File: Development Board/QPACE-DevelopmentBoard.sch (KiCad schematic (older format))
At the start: 25 parts, among them J1 Barrel_Jack_Switch, J10 SWD_ext, J13 RF_External, J2 5Vin-USB, J3 Vin, J4 Vin, J5 RPi_COMPort, J6 WTC_I2C-BUS, J7 Vout, J8 Vout, J9 GPS, SW2 SW_SPDT, U1 BMG160

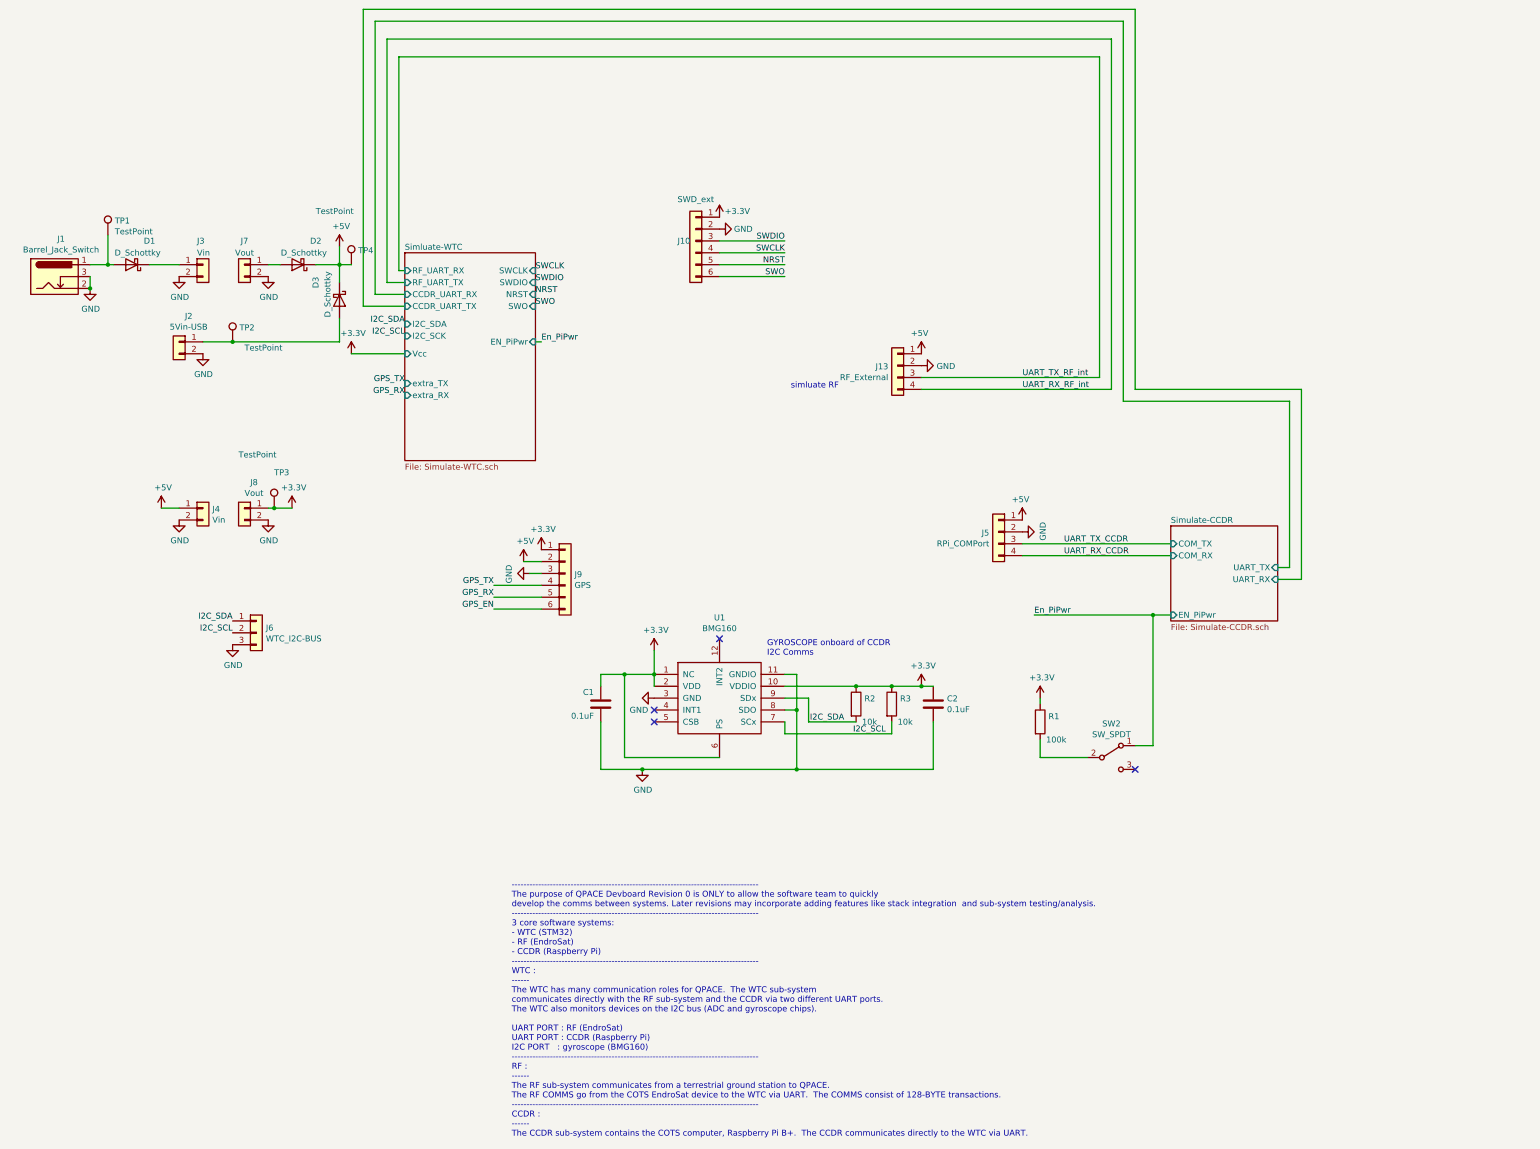
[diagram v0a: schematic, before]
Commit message: ready for production
passed all KiCad error checking. schematic and pcblayout were both validated. ready to be ordered
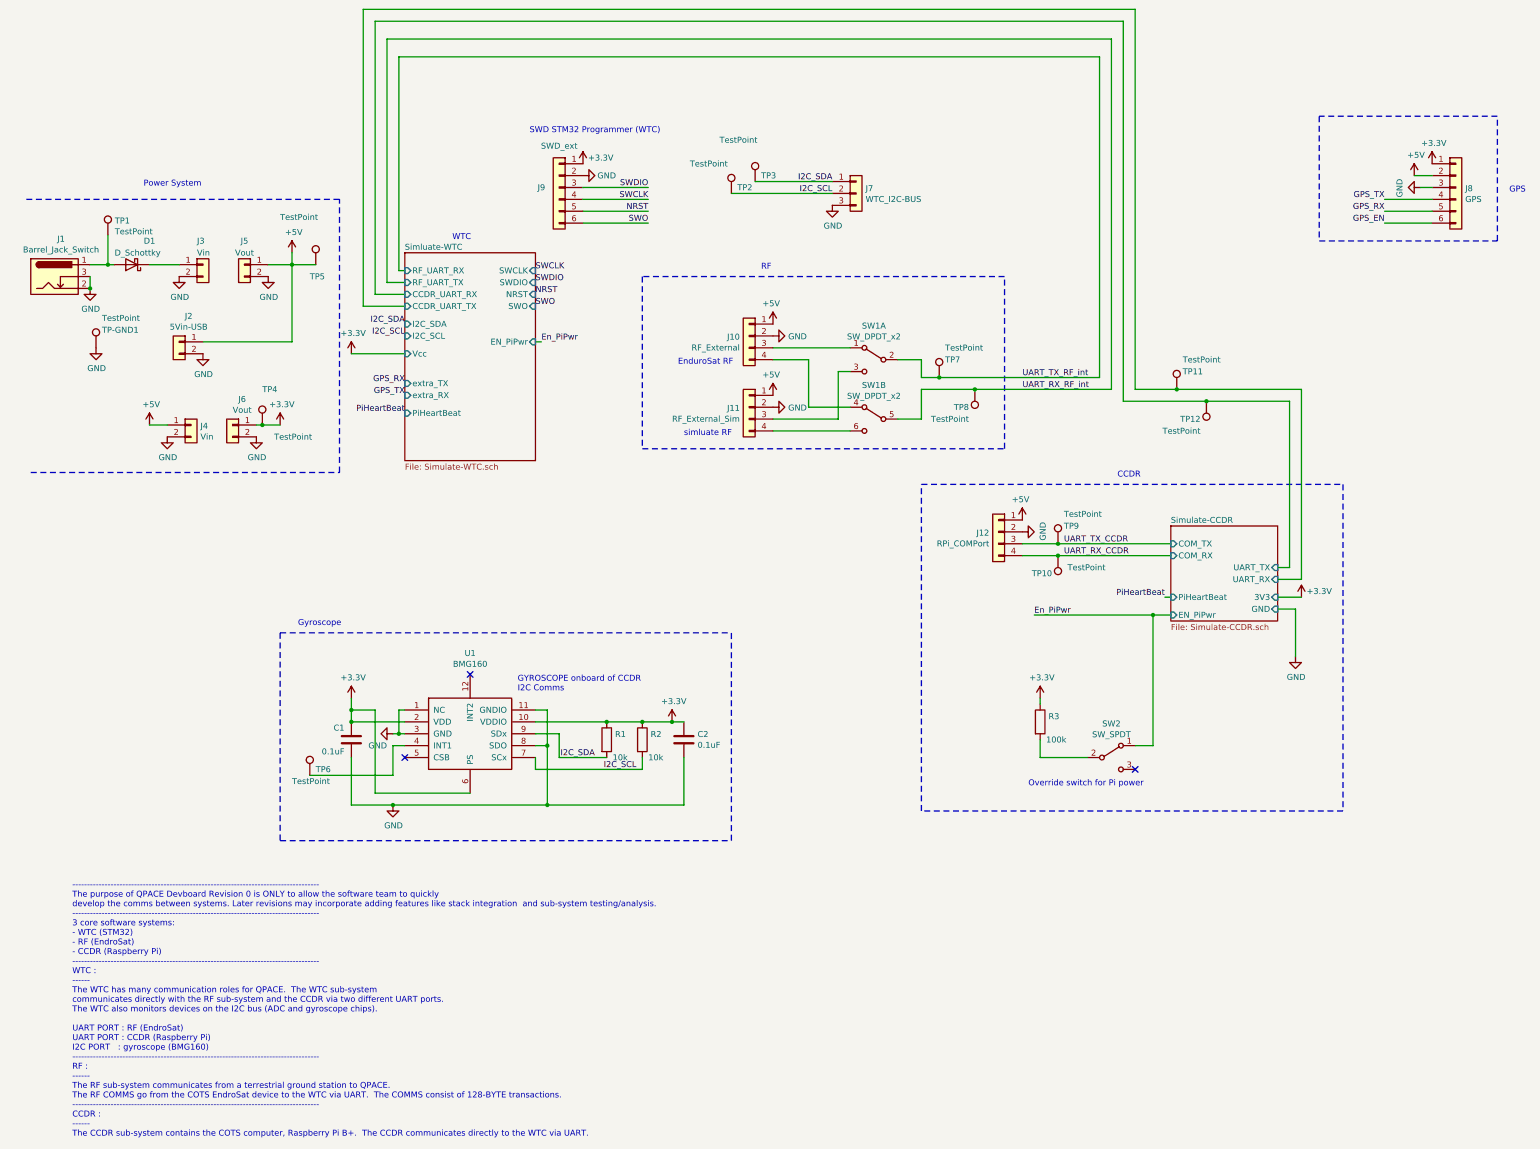
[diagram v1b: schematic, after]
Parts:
- removed D2, D3: D_Schottky, project_footprints:SOD-128, symbol Device:D_Schottky
- added J11: RF_External_Sim, Socket_Strips:Socket_Strip_Straight_1x04_Pitch2.54mm, symbol QPACE-DevelopmentBoard-rescue:Conn_01x04-conn
- added SW1: SW_DPDT_x2, project_footprints:Pin_Header_Straight_2x03_Pitch2.54mm, symbol Switch:SW_DPDT_x2
- added TP-GND1, TP10, TP11, TP12, TP3, TP6, TP7, TP8, TP9: TestPoint, Measurement_Points:Measurement_Point_Round-SMD-Pad_Small, symbol Connector:TestPoint
- J1: footprint TerminalBlocks_Phoenix:TerminalBlock_Phoenix_PT-3.5mm_2pol -> TerminalBlocks_Phoenix:TerminalBlock_Phoenix_PT-3.5mm_3pol
- renumbered J13 to J10, J5 to J12, J7 to J5, J8 to J6, J6 to J7, J9 to J8, J10 to J9, R2 to R1, R3 to R2, R1 to R3, TP3 to TP4, TP4 to TP5
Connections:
- net +3V3: no longer U1.1 (NC)
- net +5V: now also J2.1 (Pin_1), J5.1 (Pin_1), J11.1 (Pin_1)
- net GND: now also U1.1 (NC), J11.2 (Pin_2), TP-GND1.1
- net I2C_SCL: now also TP2.1
- net I2C_SDA: now also TP3.1
- net Simluate-WTC/CCDR_UART_RX: now also TP12.1
- net Simluate-WTC/CCDR_UART_TX: now also TP11.1
- net UART_RX_CCDR: now also TP10.1
- net UART_RX_RF_int: now also SW1.5 (B), TP8.1; no longer J10.4 (Pin_4)
- net UART_TX_CCDR: now also TP9.1
- net UART_TX_RF_int: now also SW1.2 (B), TP7.1; no longer J10.3 (Pin_3)
- net at U1.4 (INT1): now also TP6.1
- new net: J10.3 (Pin_3), SW1.1 (A)
- new net: J10.4 (Pin_4), SW1.4 (A)
- new net: J11.3 (Pin_3), SW1.3 (C)
- new net: J11.4 (Pin_4), SW1.6 (C)
- no-connect marks 4 -> 3
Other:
- note added: "CCDR"
- note added: "EnduroSat RF"
- note added: "GPS"
- note added: "Gyroscope"
- note added: "Override switch for Pi power"
- note added: "Power System"
- note added: "RF"
- note added: "SWD STM32 Programmer (WTC)"
- note added: "WTC"
- moved on the sheet: C1, C2, J10, J4, J6, J7, J8, J9, R1, R2, TP4, TP5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
